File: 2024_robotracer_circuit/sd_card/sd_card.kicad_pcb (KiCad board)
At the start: 2 copper layers, 11 parts, among them J1 Micro_SD_Card_Det1, J2 PH_6p

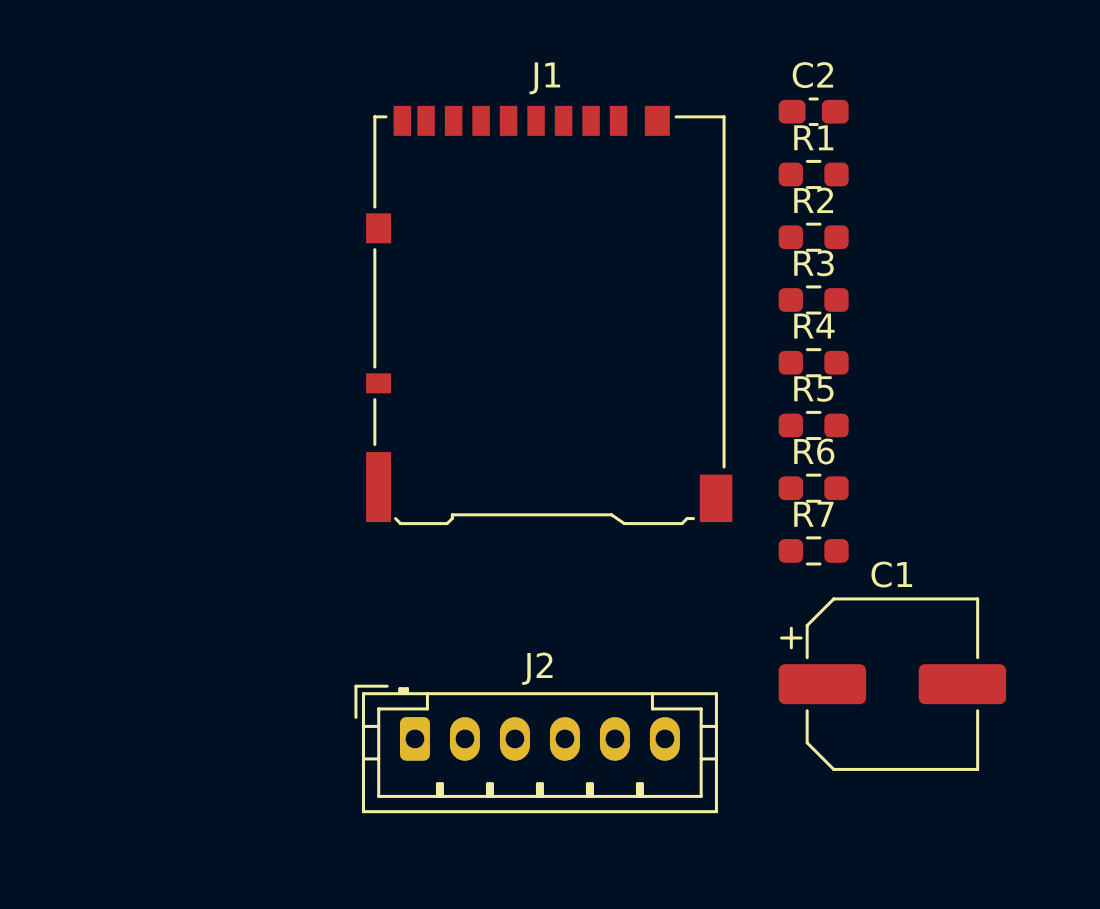
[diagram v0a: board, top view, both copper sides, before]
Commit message: sdカード
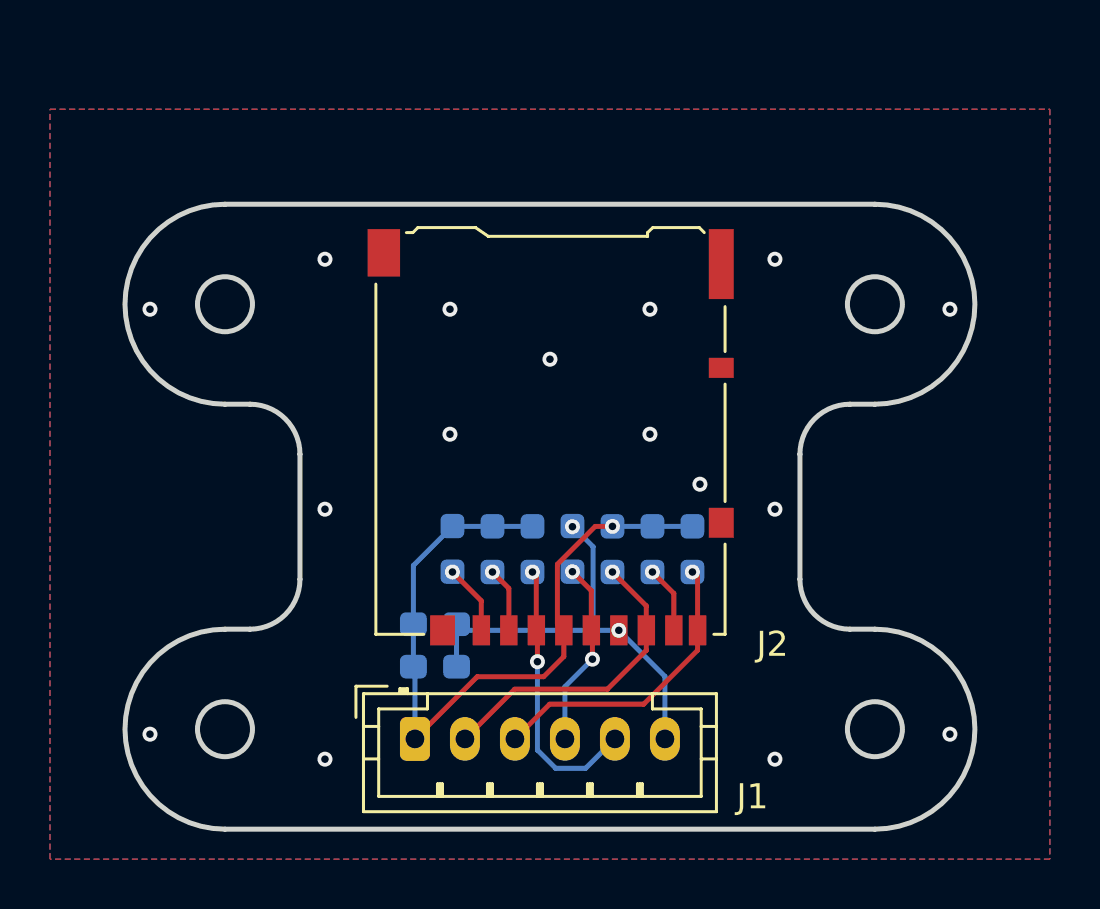
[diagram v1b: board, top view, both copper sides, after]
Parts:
- C1: value 100u -> 0.1u; footprint Capacitor_SMD:CP_Elec_6.3x5.4 -> Capacitor_SMD:C_0603_1608Metric_Pad1.08x0.95mm_HandSolder; moved to B.Cu
- C2, R1, R2, R3, R4, R5, R6, R7: moved to B.Cu
- moved C2 26.9 mm to (135.4, 102.3)
- moved R1 20.8 mm to (136.1, 97.6), turned to -90 degrees
- moved C1 18.5 mm to (135.4, 100.6)
- moved R2 17.9 mm to (137.7, 97.6), turned to -90 degrees
- moved R3 13.9 mm to (140.9, 97.6), turned to 90 degrees
- moved R4 13.5 mm to (139.3, 97.6), turned to -90 degrees
- moved R5 9.45 mm to (142.5, 97.6), turned to -90 degrees
- moved R6 6.90 mm to (144.1, 97.6), turned to -90 degrees
- moved J1 4.93 mm to (140.0, 93.1), turned to 180 degrees
- moved R7 4.85 mm to (145.7, 97.6), turned to -90 degrees
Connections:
- J2 pad 2: /SDIO_CMD -> /SDIO_D0
- J2 pad 3: /SDIO_CK -> /SDIO_SW
- J2 pad 4: /SDIO_D0 -> /SDIO_CK
- J2 pad 5: /SDIO_SW -> /SDIO_CMD
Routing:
- net +3.3V: track 0.00 -> 29.5 mm, vias 0 -> 1
- net GND: track 0.00 -> 18.0 mm, vias 0 -> 18
- net /SDIO_D0: track 0.00 -> 12.4 mm, vias 0 -> 1
- net /SDIO_SW: track 0.00 -> 12.0 mm, vias 0 -> 1
- net /SDIO_CMD: track 0.00 -> 11.1 mm, vias 0 -> 2
- net /SDIO_CK: track 0.00 -> 7.48 mm, vias 0 -> 2
- net Net-(J1-DAT2): track 0.00 -> 2.81 mm, vias 0 -> 1
- net Net-(J1-DAT1): track 0.00 -> 2.69 mm, vias 0 -> 1
- net Net-(J1-DAT3/CD): track 0.00 -> 2.60 mm, vias 0 -> 1
- added copper zone on B.Cu, net GND
- added copper zone on F.Cu, net GND
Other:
- board outline added: 34 x 25 mm
